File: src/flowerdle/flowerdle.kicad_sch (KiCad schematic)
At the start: 49 parts

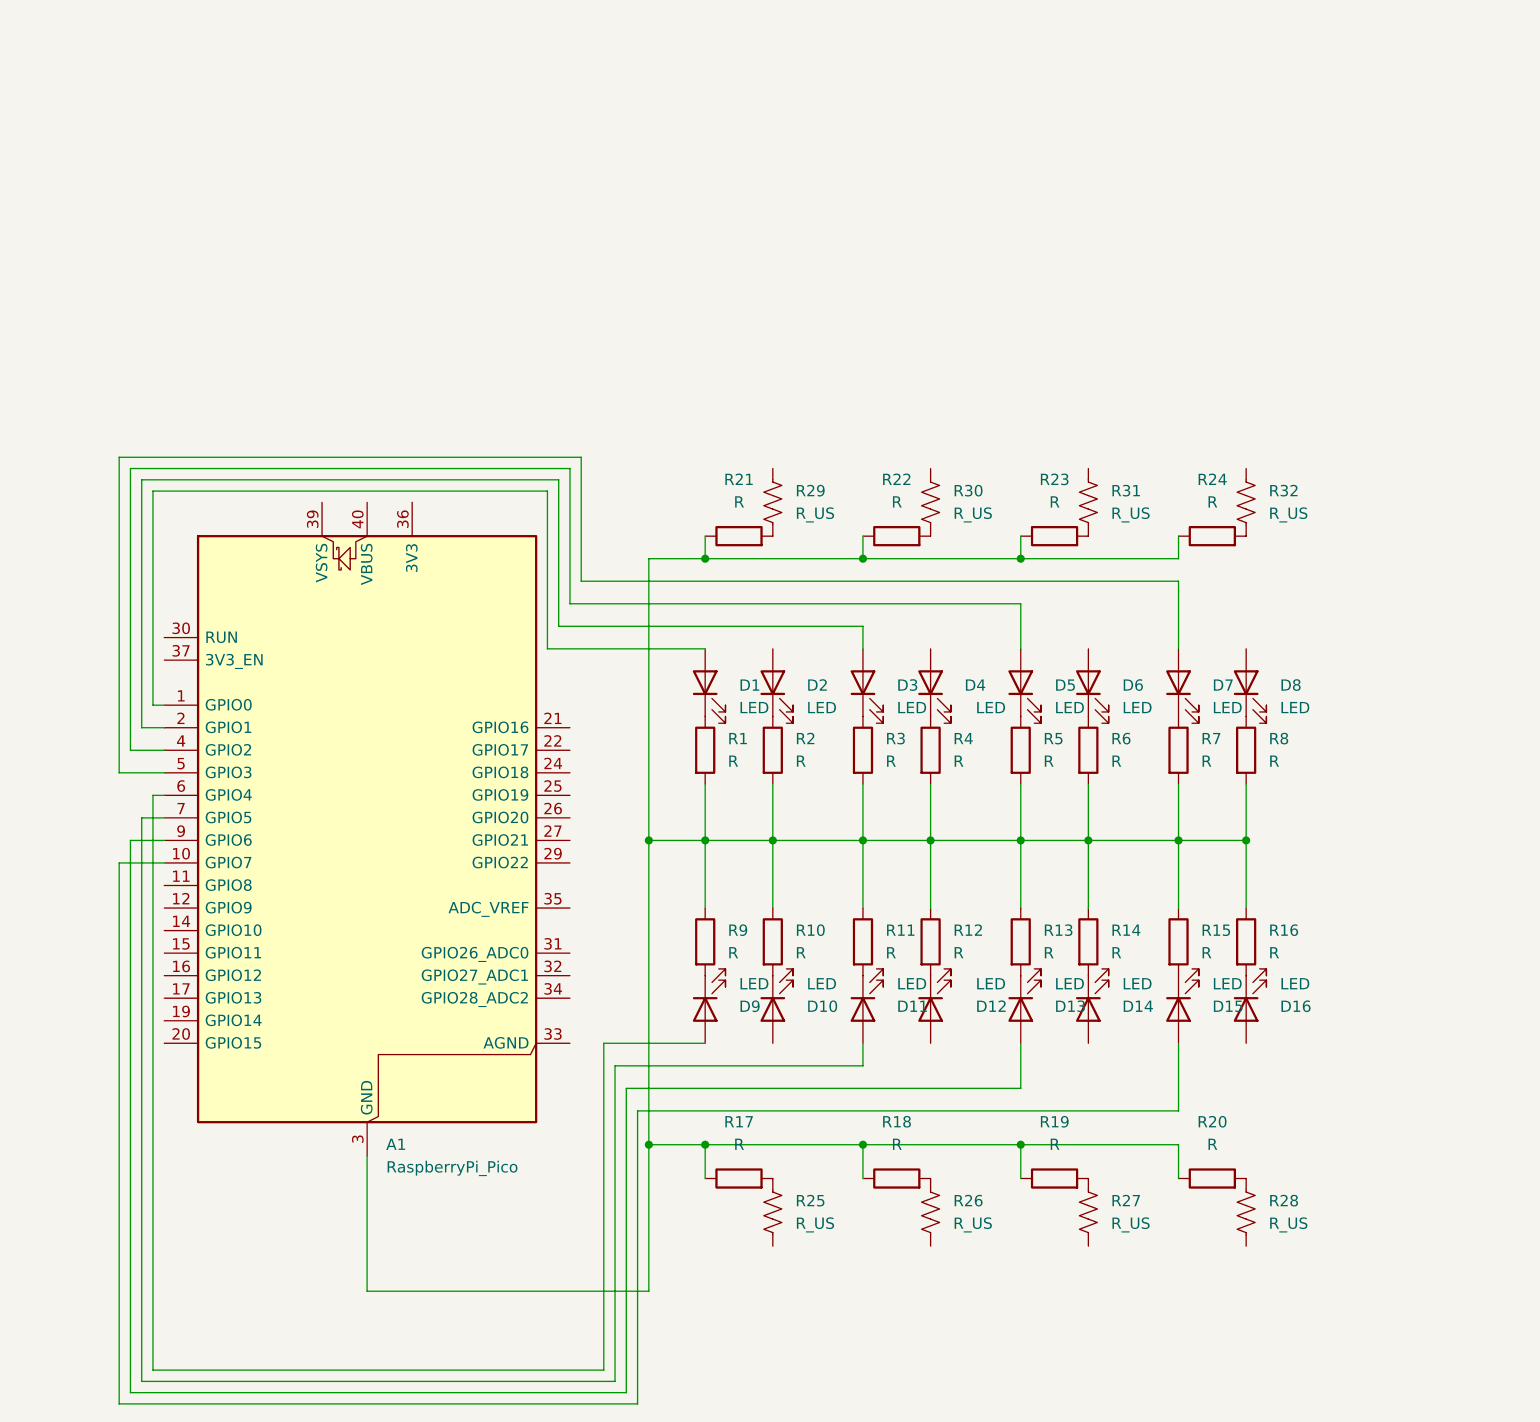
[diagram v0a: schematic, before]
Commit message: update sch
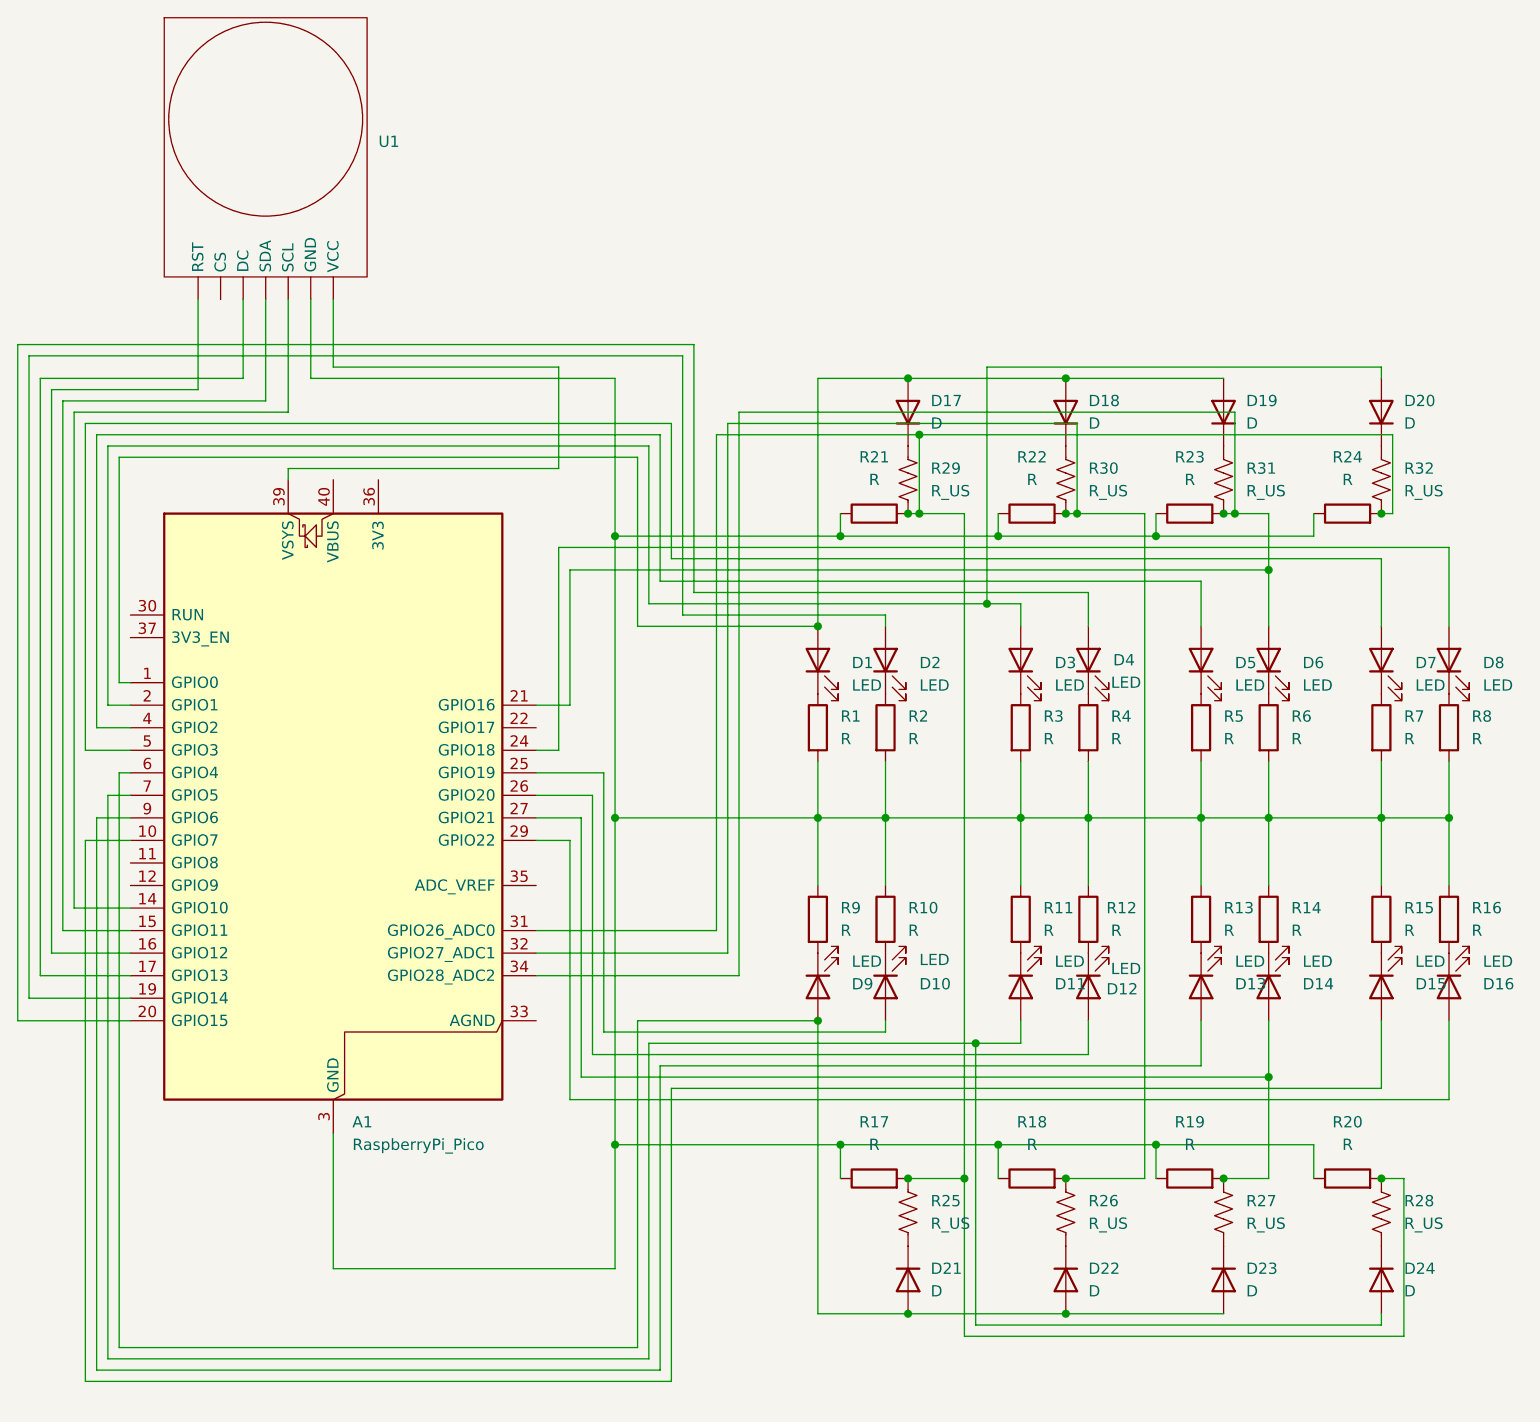
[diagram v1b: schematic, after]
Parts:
- added D17, D18, D19, D20, D21, D22, D23, D24: D, symbol Device:D
- added U1: ~, symbol KS_Maker:gc9a01
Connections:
- net at D10.2 (A): now also A1.25 (GPIO19)
- net at A1.13 (GND), A1.18 (GND), A1.23 (GND)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: now also U1. (VCC)
- net at D12.2 (A): now also A1.26 (GPIO20)
- net at R22.2, R30.2: now also A1.32 (GPIO27_ADC1), R18.2, R26.1
- net at R31.1: now also D19.1 (K)
- net at R23.2, R31.2: now also A1.21 (GPIO16), A1.34 (GPIO28_ADC2), D6.2 (A)
- net at A1.1 (GPIO0), D1.2 (A): now also D17.2 (A), D18.2 (A), D19.2 (A)
- net at A1.14 (GPIO10): now also U1. (VCC)
- net at A1.15 (GPIO11): now also U1. (VCC)
- net at A1.16 (GPIO12): now also U1. (VCC)
- net at A1.17 (GPIO13): now also U1. (VCC)
- net at A1.19 (GPIO14): now also D2.2 (A)
- net at A1.2 (GPIO1), D3.2 (A): now also D20.2 (A)
- net at A1.20 (GPIO15): now also D4.2 (A)
- net at A1.24 (GPIO18): now also D8.2 (A)
- net at A1.27 (GPIO21): now also D14.2 (A), R19.2, R27.1
- net at A1.29 (GPIO22): now also D16.2 (A)
- net at A1.31 (GPIO26_ADC0): now also R17.2, R20.2, R21.2, R24.2, R25.1, R28.1, R29.2, R32.2
- net at A1.39 (VSYS): now also U1. (VCC)
- net at A1.6 (GPIO4), D9.2 (A): now also D21.2 (A), D22.2 (A), D23.2 (A)
- net at A1.7 (GPIO5), D11.2 (A): now also D24.2 (A)
- net at R32.1: now also D20.1 (K)
- net at R29.1: now also D17.1 (K)
- net at R28.2: now also D24.1 (K)
- net at R27.2: now also D23.1 (K)
- net at R30.1: now also D18.1 (K)
- net at R26.2: now also D22.1 (K)
- net at R25.2: now also D21.1 (K)
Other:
- moved on the sheet: A1, D1, D10, D11, D12, D13, D14, D15, D16, D2, D3, D4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
